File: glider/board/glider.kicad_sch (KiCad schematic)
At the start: 9 parts, among them J1 Conn_01x05_Socket, J4 Conn_01x02, J5 Conn_01x02, U1 TPS613221ADBV 5V converter, U2 ESP32-DevKitC

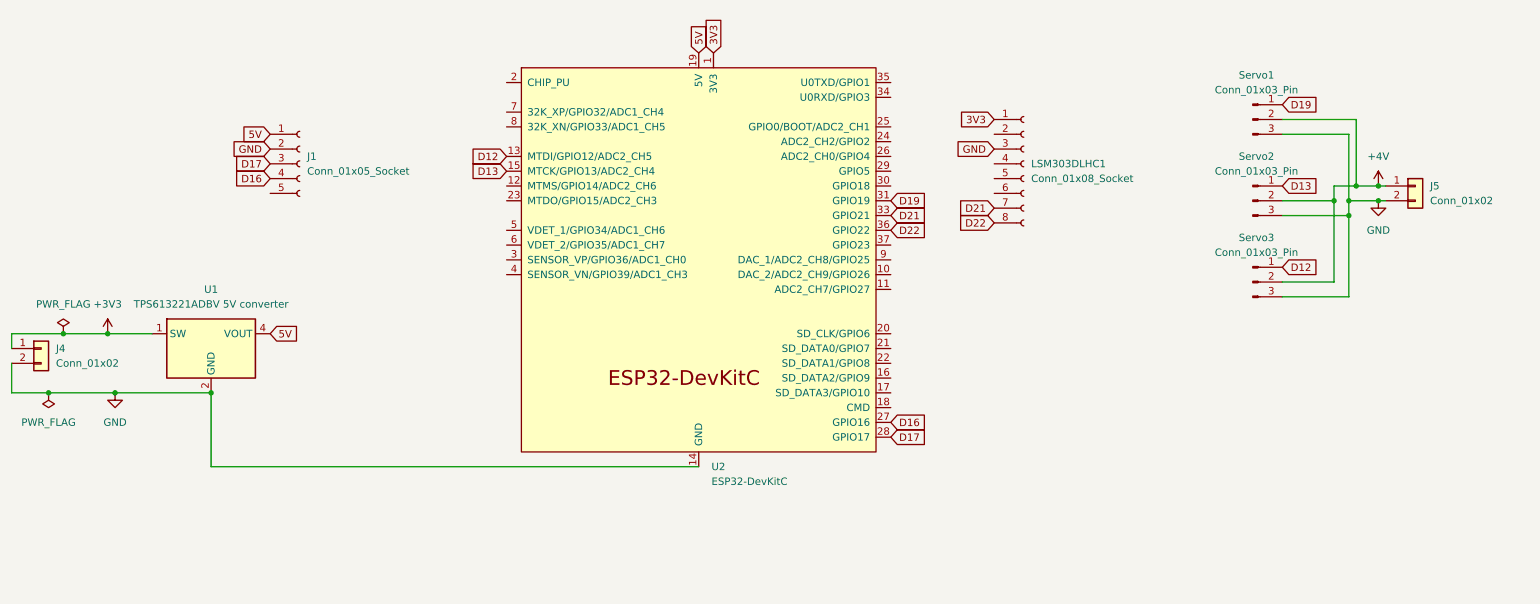
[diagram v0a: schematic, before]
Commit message: Update board
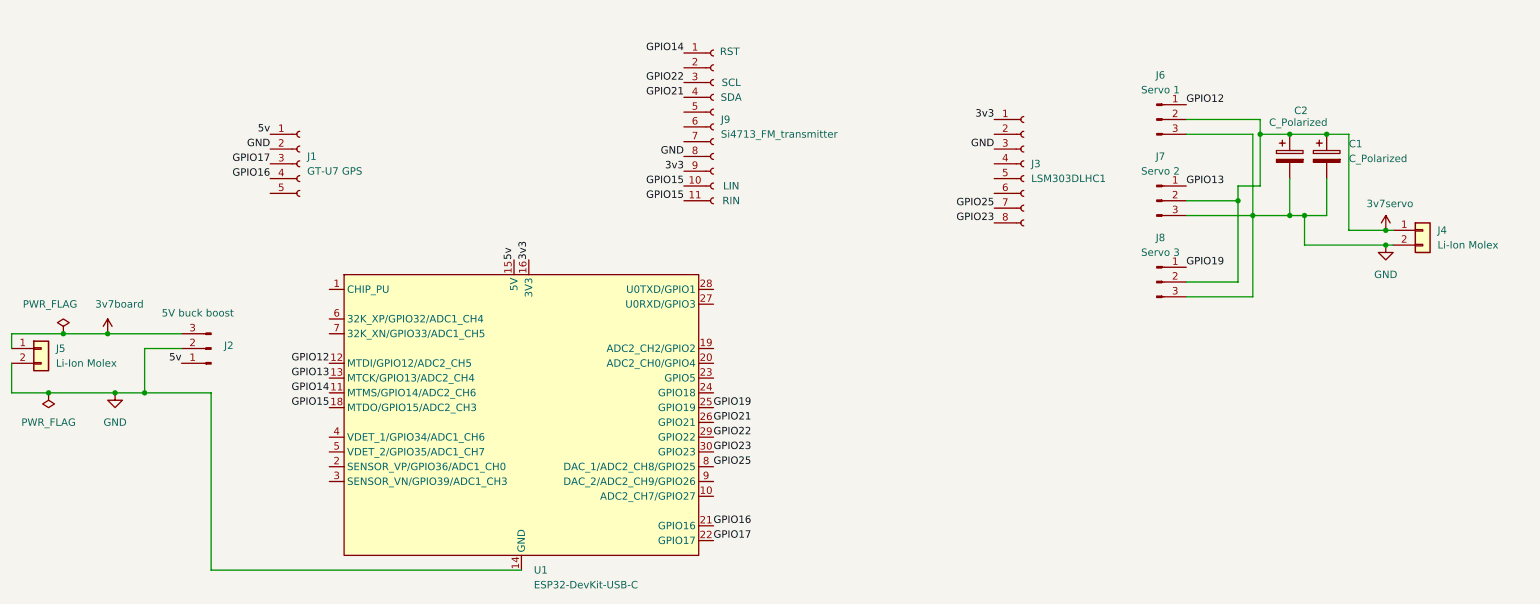
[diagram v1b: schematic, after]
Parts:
- removed U1: TPS613221ADBV 5V converter, Package_TO_SOT_SMD:SOT-23-5, symbol Regulator_Switching:TPS613221ADBV
- removed U2: ESP32-DevKitC, PCM_Espressif:ESP32-DevKitC, symbol PCM_Espressif:ESP32-DevKitC
- added C1, C2: C_Polarized, Capacitor_THT:CP_Radial_D8.0mm_P3.50mm, symbol Device:C_Polarized
- added J2: 5V buck boost, Connector_PinHeader_2.54mm:PinHeader_1x03_P2.54mm_Vertical, symbol Connector:Conn_01x03_Pin
- added J9: Si4713_FM_transmitter, Connector_PinSocket_2.54mm:PinSocket_1x11_P2.54mm_Vertical, symbol Connector:Conn_01x11_Socket
- added U1: ESP32-DevKit-USB-C, boards:ESP32-DevKit-USB-C, symbol boards:ESP32-DevKit-USB-C
- J1: value Conn_01x05_Socket -> GT-U7 GPS
- J3: renamed from LSM303DLHC1; value Conn_01x08_Socket -> LSM303DLHC1
- J4: renamed from J5; value Conn_01x02 -> Li-Ion Molex
- J5: renamed from J4; value Conn_01x02 -> Li-Ion Molex
- J6: renamed from Servo1; value Conn_01x03_Pin -> Servo 1
- J7: renamed from Servo2; value Conn_01x03_Pin -> Servo 2
- J8: renamed from Servo3; value Conn_01x03_Pin -> Servo 3
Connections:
- net GND: now also C1.2, C2.2, J2.2 (Pin_2), J9.8 (Pin_8), U1.14 (GND), U1.17 (GND)
- net +3V3 renamed 3v7board
- net 3v7board: now also J2.3 (Pin_3)
- net +4V renamed 3v7servo
- net 3v7servo: now also C1.1, C2.1
- net 3V3 renamed 3v3
- net 3v3: now also J9.9 (Pin_9), U1.16 (3V3)
- net 5V renamed 5v
- net 5v: now also J2.1 (Pin_1), U1.15 (5V)
- net D12 renamed GPIO19
- net GPIO19: now also U1.25 (GPIO19)
- net D13 renamed GPIO13
- net GPIO13: now also U1.13 (MTCK/GPIO13/ADC2_CH4)
- net D16 renamed GPIO16
- net GPIO16: now also U1.21 (GPIO16)
- net D17 renamed GPIO17
- net GPIO17: now also U1.22 (GPIO17)
- net D19 renamed GPIO12
- net GPIO12: now also U1.12 (MTDI/GPIO12/ADC2_CH5)
- net D21 renamed GPIO25
- net GPIO25: now also U1.8 (DAC_1/ADC2_CH8/GPIO25)
- net D22 renamed GPIO23
- net GPIO23: now also U1.30 (GPIO23)
- new net GPIO14: J9.1 (Pin_1), U1.11 (MTMS/GPIO14/ADC2_CH6)
- new net GPIO15: J9.10 (Pin_10), J9.11 (Pin_11), U1.18 (MTDO/GPIO15/ADC2_CH3)
- new net GPIO21: J9.4 (Pin_4), U1.26 (GPIO21)
- new net GPIO22: J9.3 (Pin_3), U1.29 (GPIO22)
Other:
- note added: "LIN"
- note added: "RIN"
- note added: "RST"
- note added: "SCL"
- note added: "SDA"
- moved on the sheet: J4, J6, J7, J8
